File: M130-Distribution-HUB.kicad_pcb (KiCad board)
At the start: 4 copper layers, 152.4 x 114.3 mm, 23 parts, among them CN0 6437288-3

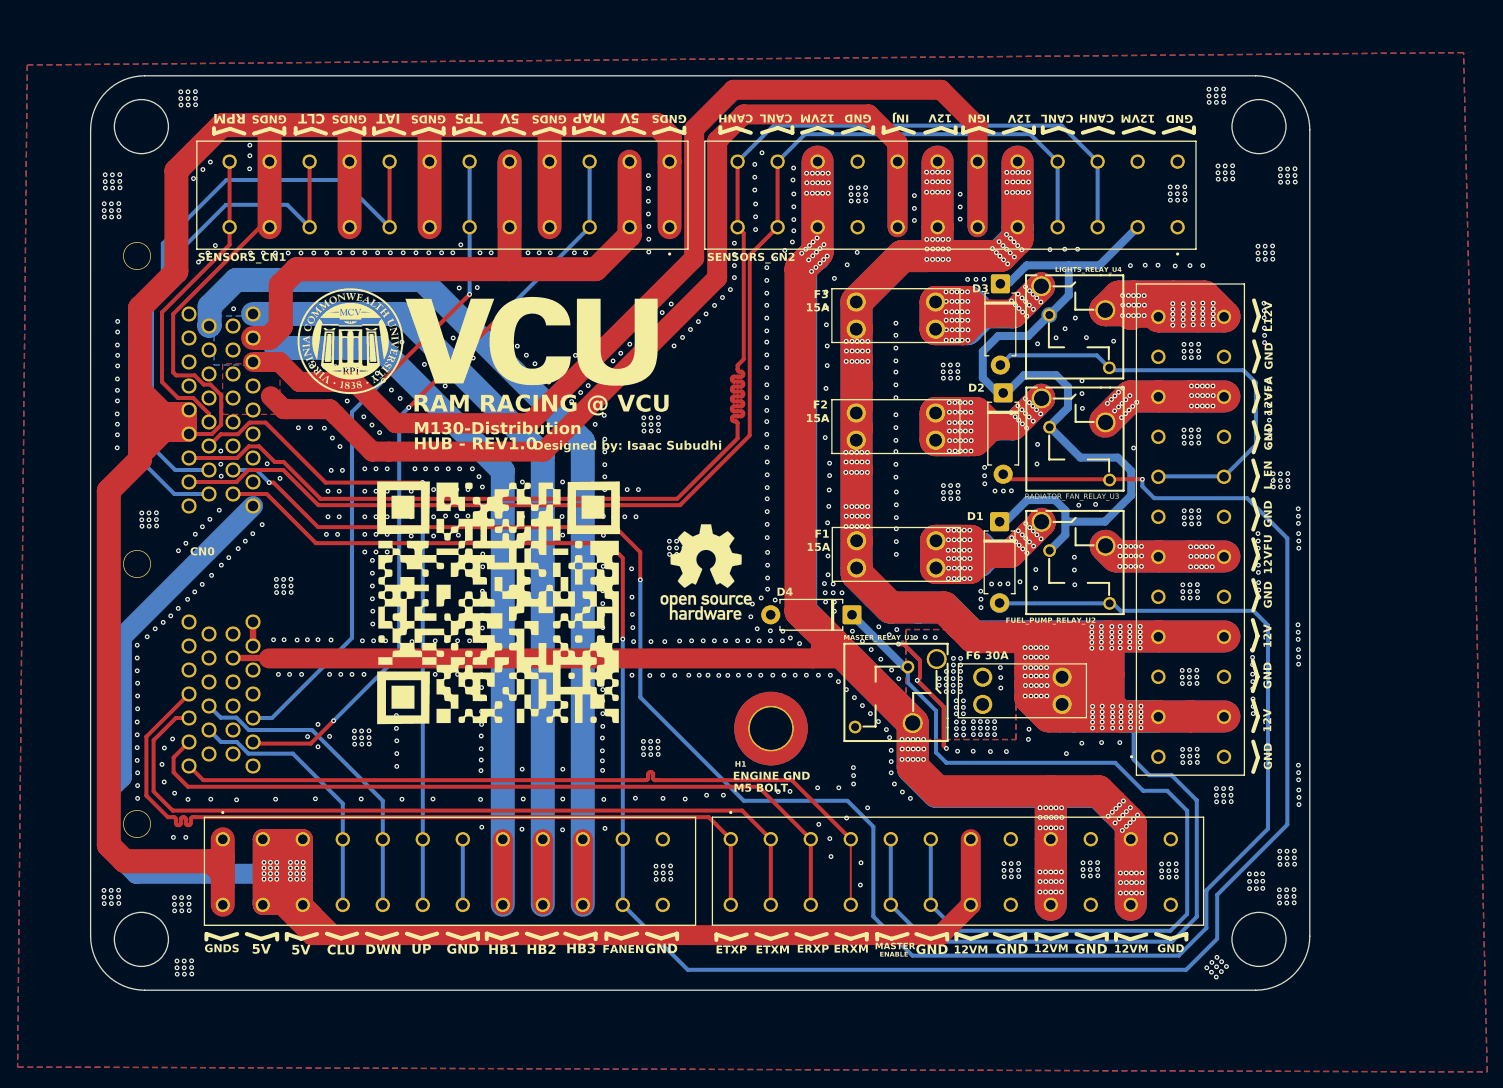
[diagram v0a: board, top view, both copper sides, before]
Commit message: Slight changes
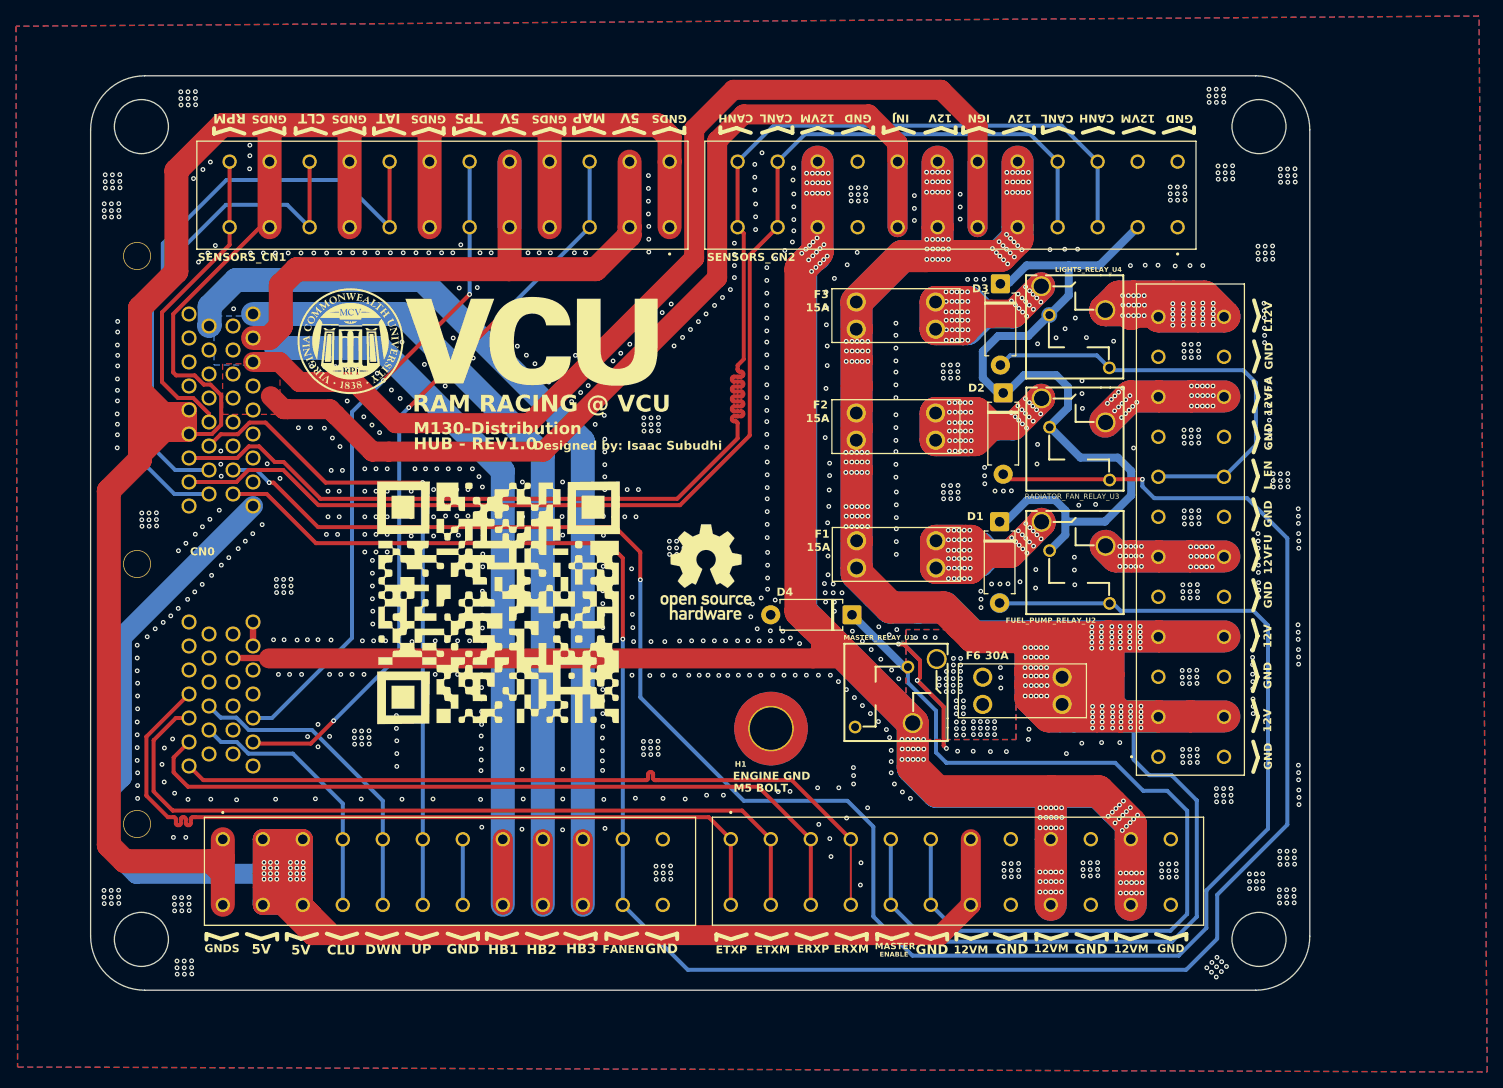
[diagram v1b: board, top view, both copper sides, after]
